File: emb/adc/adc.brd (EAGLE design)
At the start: 100 x 80 mm, 21 parts, among them IC1 AD623N, IC2 MCP3008, Q1 RD06HVF1, Q2 RD06HVF1, Q3 RD06HVF1, Q4 RD06HVF1

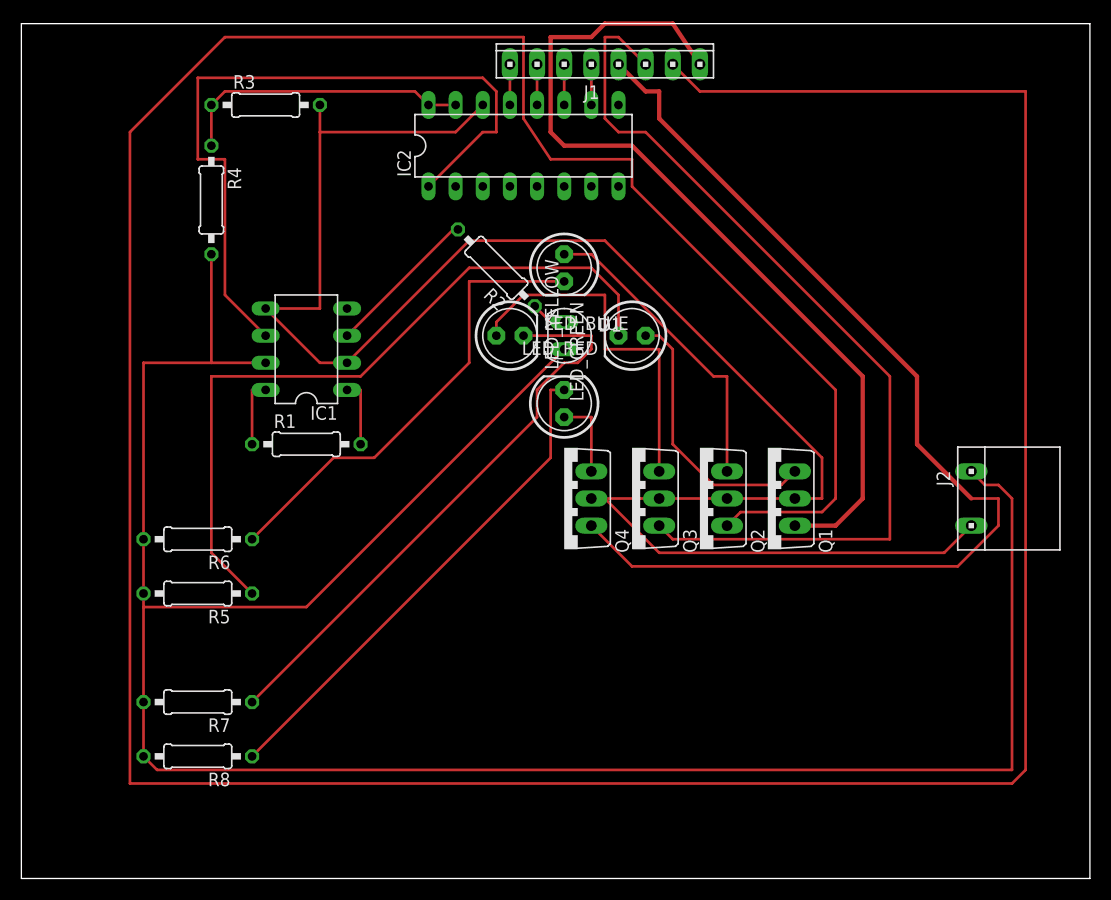
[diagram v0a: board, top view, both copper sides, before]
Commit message: new board
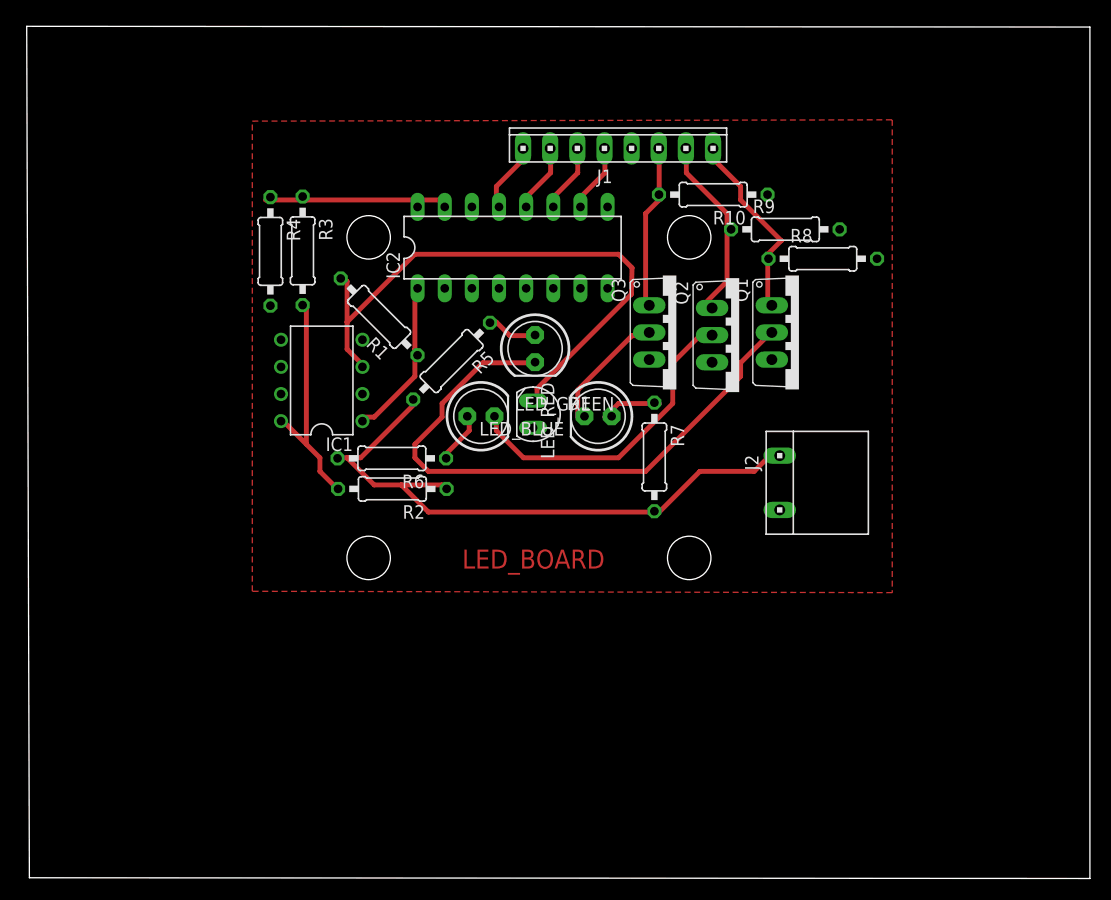
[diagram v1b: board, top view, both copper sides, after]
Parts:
- removed LED_YELLOW: (no value), adafruit:LED5MM
- removed Q4: RD06HVF1, transistor-power:RD06HVF1
- added R10, R9: 12K, rcl:0207/10
- IC1: value AD623N -> LM358N; device analog-devices:DIL08 -> linear:DIL08
- Q1, Q2, Q3: value RD06HVF1 -> (none); device transistor-power:RD06HVF1 -> adafruit:TO220V
- R1: value (none) -> 100K
- R2: value (none) -> 7.5K
- R3: value (none) -> 1.2K
- R4: value (none) -> 3.3K
- R5: value (none) -> 200
- R6, R7: value (none) -> 160
- R8: value (none) -> 12K
- moved R8 74.8 mm to (75.0, 58.0), turned to 0 degrees
- moved R7 48.5 mm to (59.2, 39.5), turned to 270 degrees
- moved R5 32.2 mm to (40.3, 48.4), turned to 225 degrees
- moved R2 22.9 mm to (34.7, 36.5), turned to 180 degrees
- moved R6 19.7 mm to (34.7, 39.3)
- moved J2 18.0 mm to (71.0, 37.0)
- moved Q3 16.1 mm to (61.3, 51.1), turned to 270 degrees
- moved LED_GREEN 15.9 mm to (43.0, 43.3), turned to 0 degrees
- moved Q1 15.8 mm to (72.8, 51.1), turned to 270 degrees
- moved Q2 15.7 mm to (67.2, 50.9), turned to 270 degrees
- moved R3 14.1 mm to (26.3, 58.7), turned to 270 degrees
- moved R1 13.7 mm to (33.5, 52.6), turned to 135 degrees
- moved LED_BLUE 11.2 mm to (54.0, 43.3), turned to 180 degrees
- moved IC2 9.59 mm to (46.0, 59.0)
- moved LED_RED 9.15 mm to (48.1, 49.6), turned to 270 degrees
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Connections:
- net N$12 renamed 3.3V
- removed net -V: IC1.4
- removed net L_Y: J1.4, Q4.1
- removed net N$14: LED_RED.A, Q1.3
- removed net N$16: LED_GREEN.K, R6.1
- removed net N$17: LED_GREEN.A, Q2.3
- removed net N$18: LED_BLUE.K, R7.1
- removed net N$19: LED_YELLOW.K, R8.1
- removed net N$20: LED_BLUE.A, Q3.3
- removed net N$21: LED_YELLOW.A, Q4.3
- removed net VCC: IC2.9
- new net 4.5V: IC1.8, R2.2, R3.2
- new net N$12: LED_GREEN.A, R6.1
- new net N$8: LED_BLUE.A, R7.1
- net 0V: now also D1.A, IC1.4, IC2.9, Q1.3, Q2.3, Q3.3, R10.1, R4.2, R8.2, R9.2; no longer IC1.5, Q1.2, Q2.2, Q3.2, Q4.2, R3.2
- net 12V: now also R2.1; no longer D1.A, IC1.7, R4.2, R8.2
- net L_B: now also R10.2
- net L_G: now also R9.1
- net L_R: now also R8.1
- net N$1: now also D1.K, IC1.3; no longer IC1.1
- net N$13: now also LED_GREEN.K, Q2.2; no longer LED_RED.K, R5.1
- net N$2: now also LED_BLUE.K, Q3.2; no longer IC1.8, R1.1
- net N$3: now also LED_RED.A, R5.1; no longer D1.K, R2.1
- net N$6: now also LED_RED.K, Q1.2; no longer IC1.3, R2.2
- net N$7: now also IC1.1, R1.1; no longer IC1.6
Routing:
- net L_G: track 354.1 -> 19.2 mm
- net 0V: track 170.6 -> 0.00 mm
- net 12V: track 219.9 -> 60.1 mm
- net L_Y: track 101.4 -> 0.00 mm
- net L_B: track 86.5 -> 16.5 mm
- net L_R: track 82.9 -> 19.1 mm
- net N$18: track 54.5 -> 0.00 mm
- net N$7: track 69.0 -> 16.0 mm
- net N$1: track 6.35 -> 55.9 mm
- net N$19: track 47.1 -> 0.00 mm
- net N$16: track 43.7 -> 0.00 mm
- net N$6: track 14.7 -> 56.8 mm
- net N$13: track 69.1 -> 29.7 mm
- net N$20: track 34.1 -> 0.00 mm
- net N$17: track 28.9 -> 0.00 mm
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- added copper zone on layer 1, net 0V
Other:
- board size 100 x 80 mm -> 99.5 x 79.8 mm
- board text added: "LED_BOARD"
